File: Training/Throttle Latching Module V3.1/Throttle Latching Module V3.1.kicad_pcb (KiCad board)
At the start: 2 copper layers, 46 x 25 mm, 0 parts

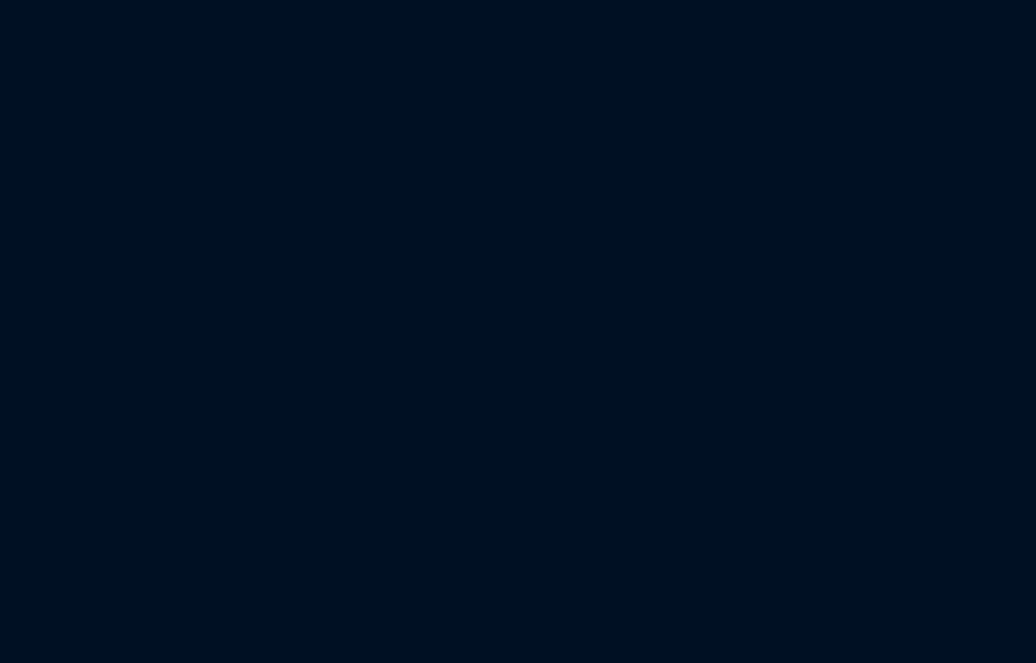
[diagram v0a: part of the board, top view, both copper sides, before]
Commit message: changes
changes
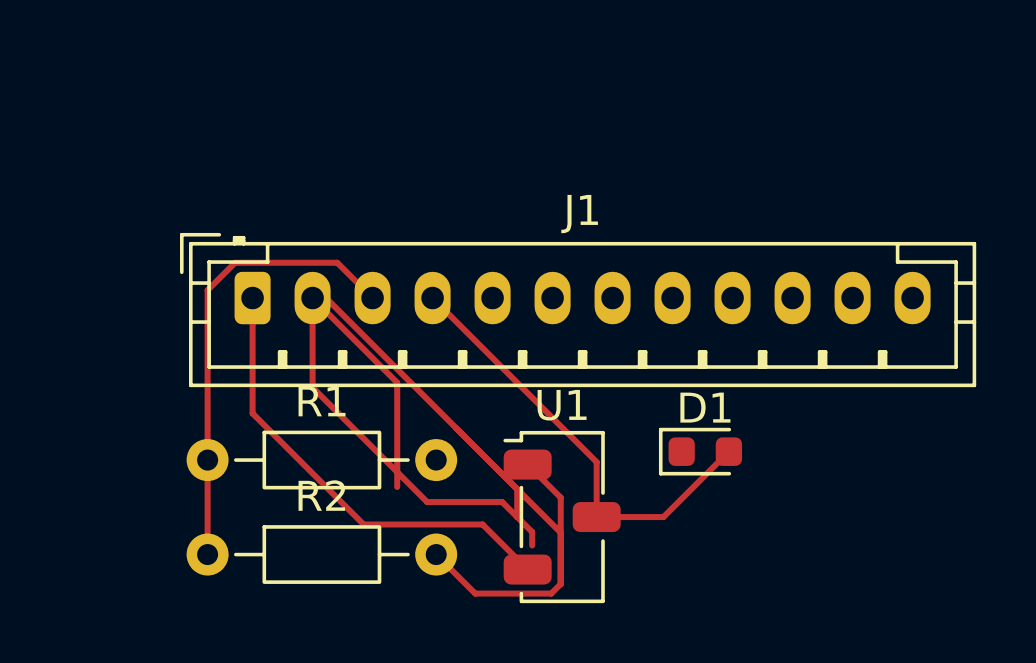
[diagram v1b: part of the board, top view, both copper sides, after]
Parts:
- added D1: LED (Test), LED_SMD:LED_0603_1608Metric, F.Cu at (156.8, 96.3)
- added J1: PH1-10-UA, Connector_JST:JST_PH_B12B-PH-K_1x12_P2.00mm_Vertical, F.Cu at (141.7, 91.2)
- added R1: 150R, Resistor_THT:R_Axial_DIN0204_L3.6mm_D1.6mm_P7.62mm_Horizontal, F.Cu at (140.2, 96.6)
- added R2: 10k, Resistor_THT:R_Axial_DIN0204_L3.6mm_D1.6mm_P7.62mm_Horizontal, F.Cu at (140.2, 99.8)
- added U1: IRLML2060TRPBF, Button_Switch_SMD:Nidec_Copal_CAS-120A, F.Cu at (152.0, 98.5)
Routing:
- net Net-(U1-G): track 0.00 -> 47.3 mm
- net Net-(U1-D): track 0.00 -> 15.5 mm
- net Net-(J1-Pad3): track 0.00 -> 15.2 mm
- net Net-(D1-A): track 0.00 -> 15.0 mm
- net Net-(D1-K): track 0.00 -> 0.65 mm

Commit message: Revert "changes"
This reverts commit 10df18be739a6716873fb9f13ef638a2302d6145.
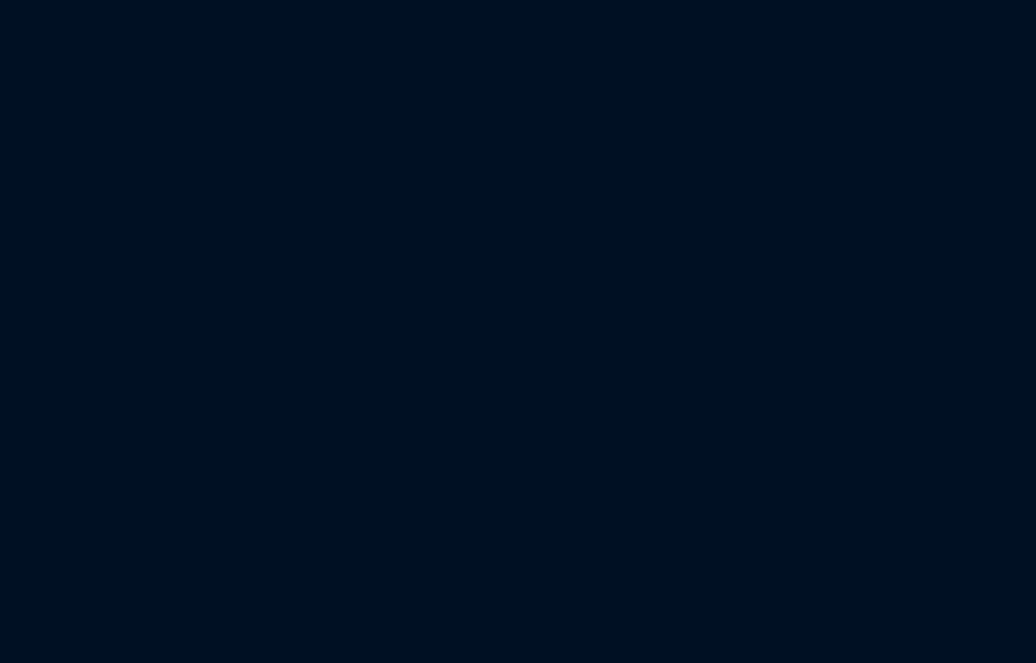
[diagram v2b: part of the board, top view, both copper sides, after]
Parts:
- removed D1: LED (Test), LED_SMD:LED_0603_1608Metric
- removed J1: PH1-10-UA, Connector_JST:JST_PH_B12B-PH-K_1x12_P2.00mm_Vertical
- removed R1: 150R, Resistor_THT:R_Axial_DIN0204_L3.6mm_D1.6mm_P7.62mm_Horizontal
- removed R2: 10k, Resistor_THT:R_Axial_DIN0204_L3.6mm_D1.6mm_P7.62mm_Horizontal
- removed U1: IRLML2060TRPBF, Button_Switch_SMD:Nidec_Copal_CAS-120A
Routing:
- net Net-(U1-G): track 47.3 -> 0.00 mm
- net Net-(U1-D): track 15.5 -> 0.00 mm
- net Net-(J1-Pad3): track 15.2 -> 0.00 mm
- net Net-(D1-A): track 15.0 -> 0.00 mm
- net Net-(D1-K): track 0.65 -> 0.00 mm
